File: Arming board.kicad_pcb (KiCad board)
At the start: 2 copper layers, 43.5 x 46.3 mm, 26 parts, among them IC1 CD4043BDR, J3 Conn_01x04, Q1 SQS141ELNW-T1_GE3

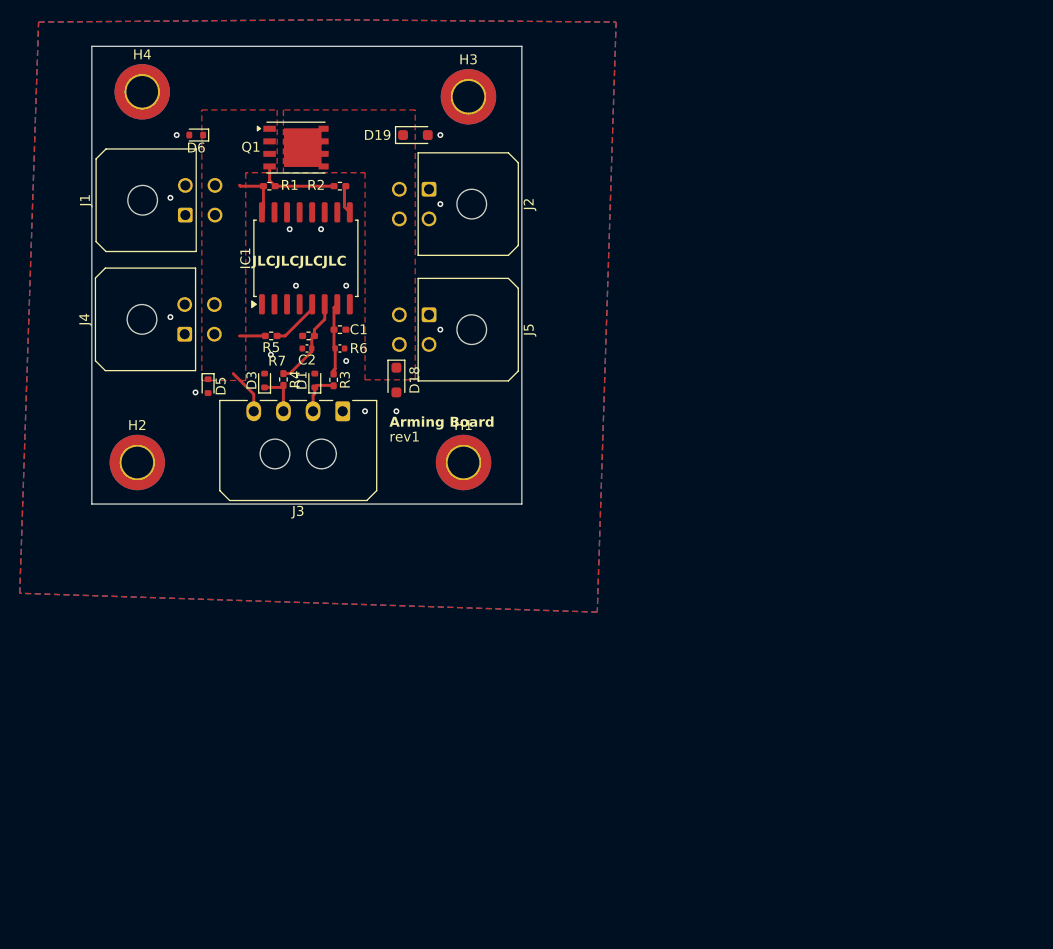
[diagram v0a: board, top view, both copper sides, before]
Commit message: improve routing
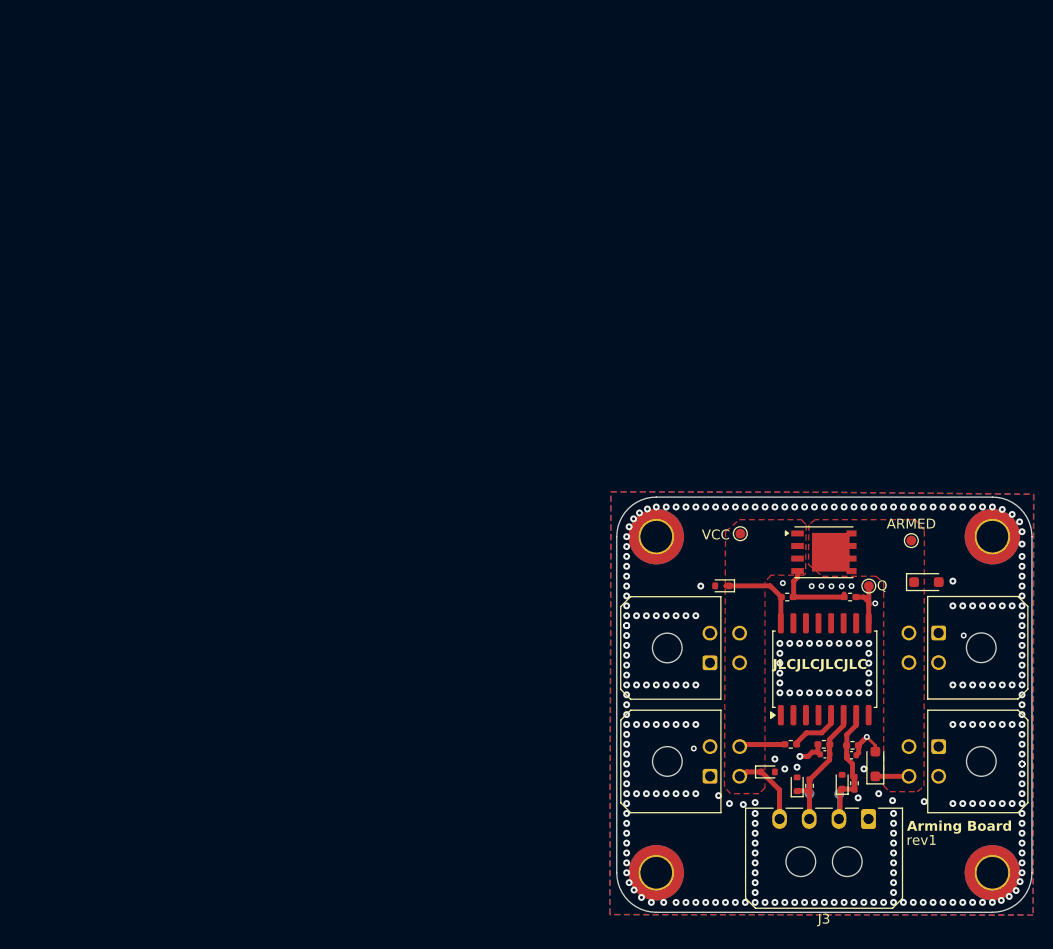
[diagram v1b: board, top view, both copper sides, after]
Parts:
- added G***: LOGO, frodo_io_module:rapid_logo, B.Cu at (129.6, 122.8)
- added TP1: TestPoint, TestPoint:TestPoint_Pad_D1.0mm, F.Cu at (140.5, 125.0)
- added TP2: TestPoint, TestPoint:TestPoint_Pad_D1.0mm, B.Cu at (137.5, 146.0)
- added TP3: TestPoint, TestPoint:TestPoint_Pad_D1.0mm, B.Cu at (134.5, 146.0)
- added TP4: TestPoint, TestPoint:TestPoint_Pad_D1.0mm, F.Cu at (127.5, 119.7)
- added TP5: TestPoint, TestPoint:TestPoint_Pad_D1.0mm, F.Cu at (144.8, 120.4)
- moved H3 94.7 mm to (153.0, 154.0)
- moved H4 94.6 mm to (119.0, 154.0)
- moved D6 70.1 mm to (125.7, 125.0)
- moved J1 69.8 mm to (124.4, 132.8)
- moved J4 69.5 mm to (124.4, 144.2)
- moved D5 68.8 mm to (130.3, 143.8), turned to 0 degrees
- moved D19 68.7 mm to (146.3, 124.6)
- moved J2 68.3 mm to (147.6, 129.7)
- moved D3 67.6 mm to (133.2, 145.1)
- moved J5 67.6 mm to (147.6, 141.2)
- moved J3 67.3 mm to (140.5, 148.6)
- moved Q1 67.3 mm to (136.0, 121.6)
- moved R4 67.2 mm to (134.5, 145.2)
- moved D1 67.0 mm to (137.8, 144.8)
- moved IC1 67.0 mm to (136.0, 133.4)
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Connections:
- D1 pad 1: Net-(D1-K) -> arm
- D3 pad 1: Net-(D3-K) -> disarm
- J3 pad 2: Net-(D1-K) -> arm
- J3 pad 3: Net-(D3-K) -> disarm
- R3 pad 2: Net-(D1-K) -> arm
- R4 pad 2: Net-(D3-K) -> disarm
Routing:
- net VCC: track 12.5 -> 21.3 mm
- net disarm: track 9.11 -> 17.8 mm
- net arm: track 7.30 -> 15.5 mm
- net GND: track 0.00 -> 7.27 mm, vias 15 -> 283
- net Net-(D3-K): track 4.60 -> 0.00 mm
- net Net-(D1-K): track 4.49 -> 0.00 mm
- net +BATT_ARM: track 0.00 -> 3.21 mm
- net Net-(IC1-Q2): track 2.93 -> 5.58 mm
- net Net-(IC1-ENABLE): track 5.14 -> 6.14 mm
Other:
- board size 43.5 x 46.3 mm -> 42 x 42 mm
- board text added: "ARM"
- board text added: "ARMED"
- board text added: "DISARM"
- board text added: "GND"
- board text added: "Power In"
- board text added: "Power Out"
- board text added: "Q"
- board text added: "VCC"
